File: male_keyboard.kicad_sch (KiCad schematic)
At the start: 1 part, among them J1 Elite-Pi Microcontroller

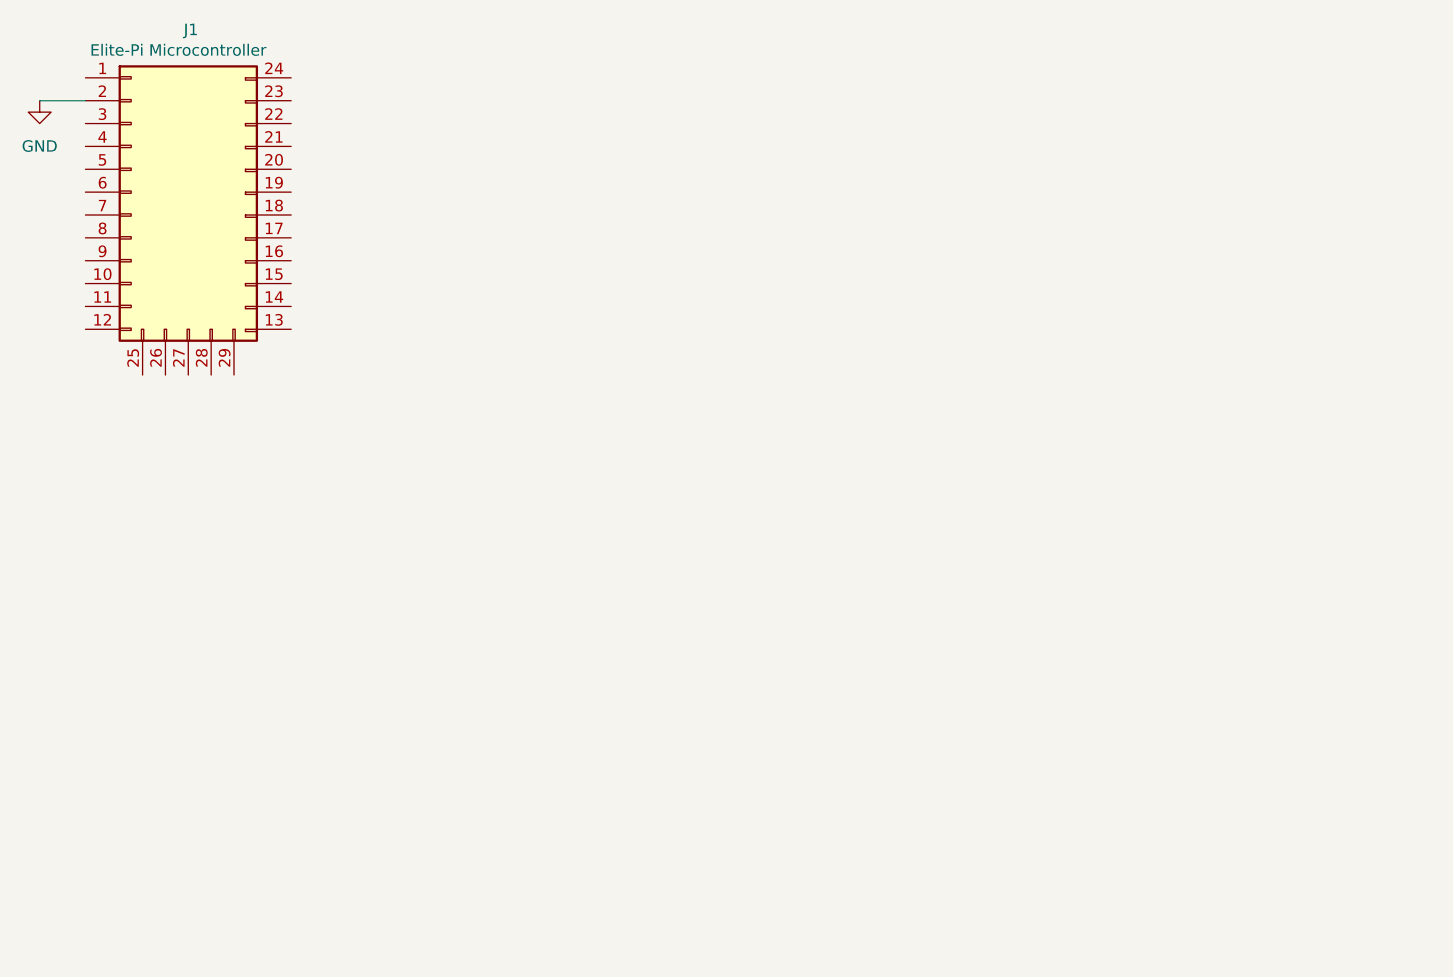
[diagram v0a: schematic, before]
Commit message: 1504202502
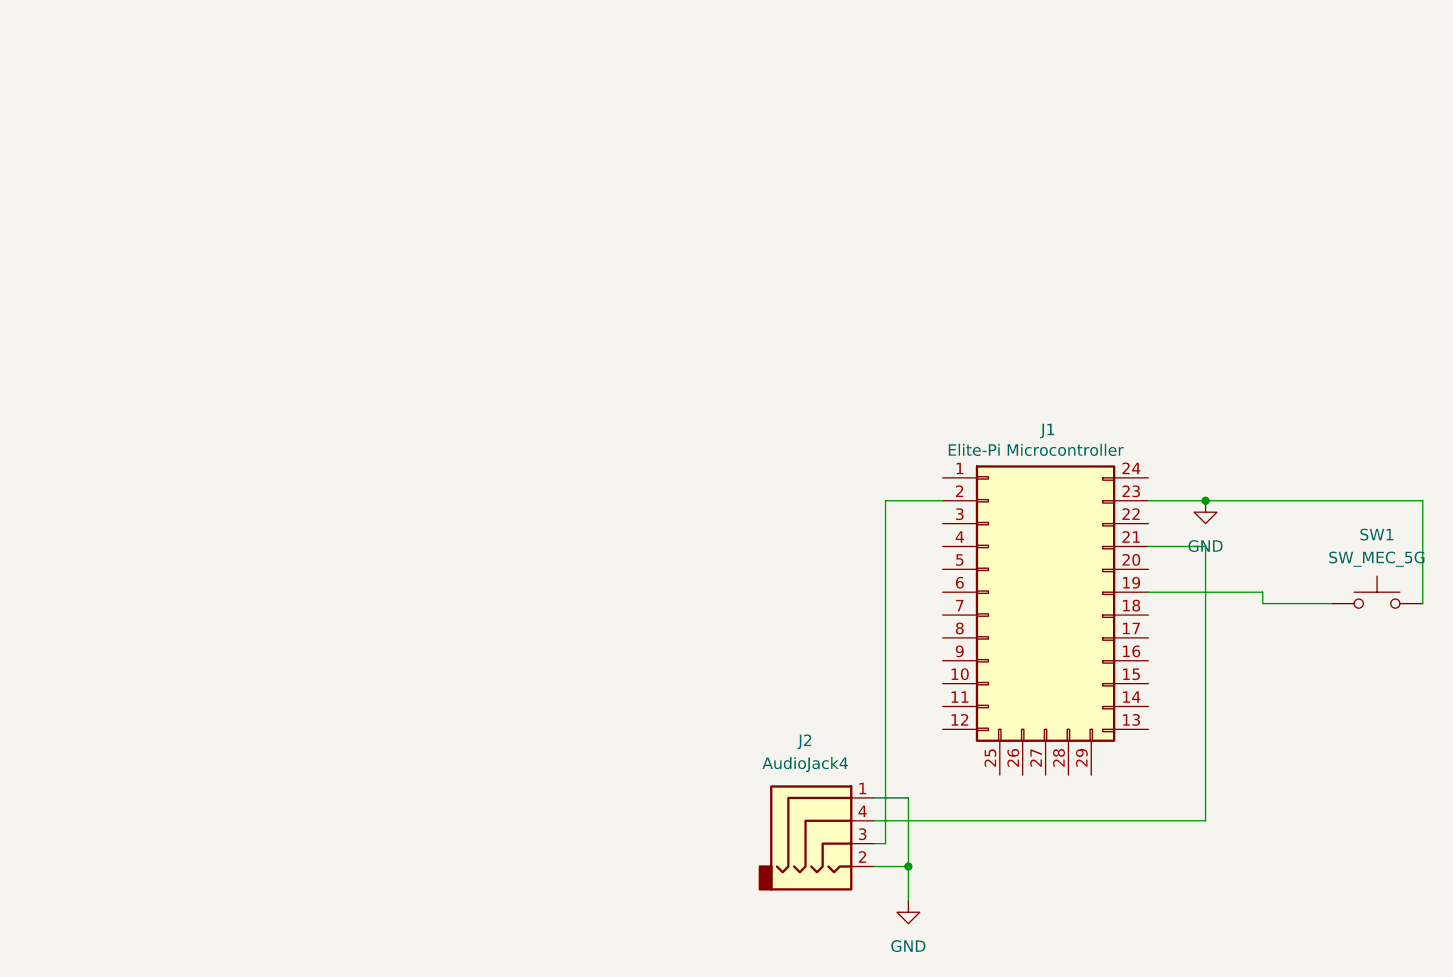
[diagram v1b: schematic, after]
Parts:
- added J2: AudioJack4, Keebio-Parts:TRRS-PJ-320A, symbol Connector_Audio:AudioJack4
- added SW1: SW_MEC_5G, Button_Switch_Keyboard:SW_Cherry_MX_1.00u_PCB, symbol Switch:SW_MEC_5G
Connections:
- net GND: now also J1.23 (Pin_23), J2.1, J2.2, SW1.2; no longer J1.2 (Pin_2)
- net at J1.19 (Pin_19): now also SW1.1
- net at J1.21 (Pin_21): now also J2.4
- new net: J1.2 (Pin_2), J2.3
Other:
- moved on the sheet: J1
